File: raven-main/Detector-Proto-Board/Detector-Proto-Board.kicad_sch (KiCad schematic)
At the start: 17 parts, among them IC1 ADA4817-1ARDZ-R7, J1 Conn_01x04, U9 TLV3201AIDCKT

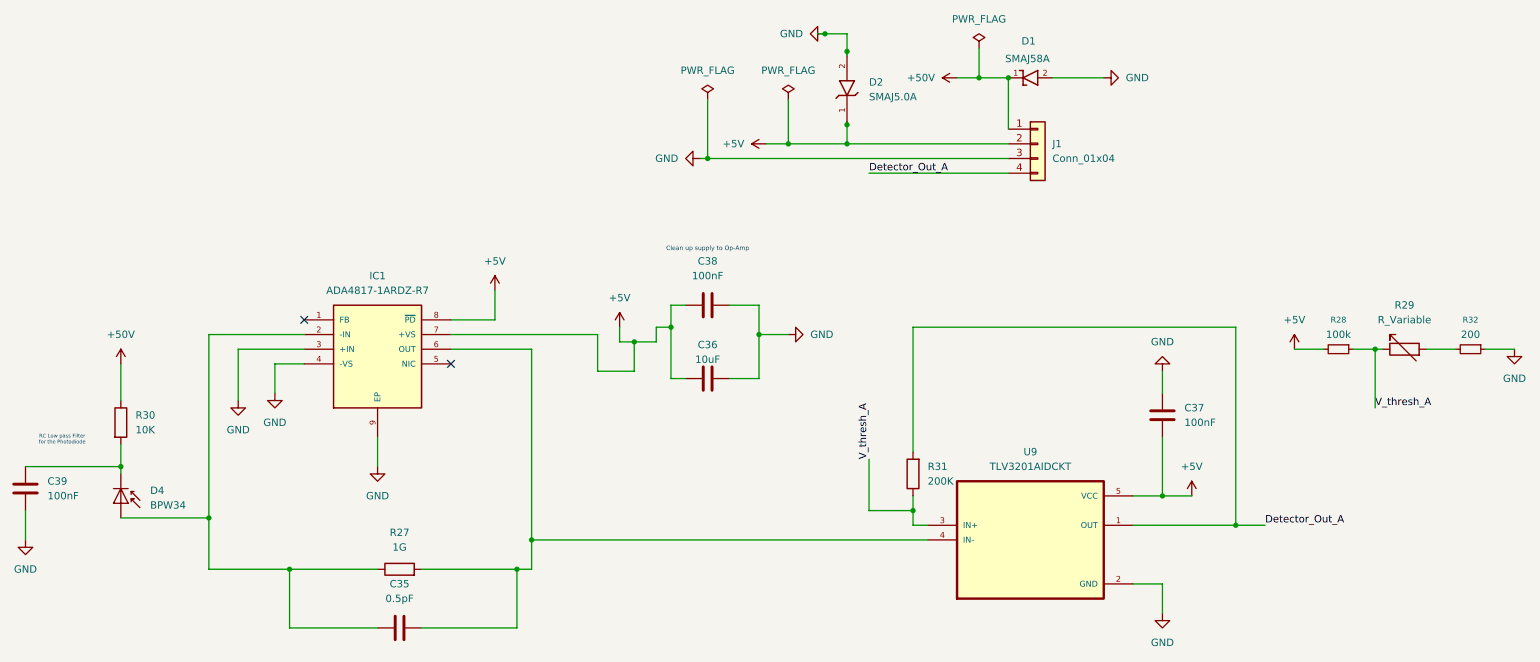
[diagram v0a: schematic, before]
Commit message: feat:PCB layout changes - example
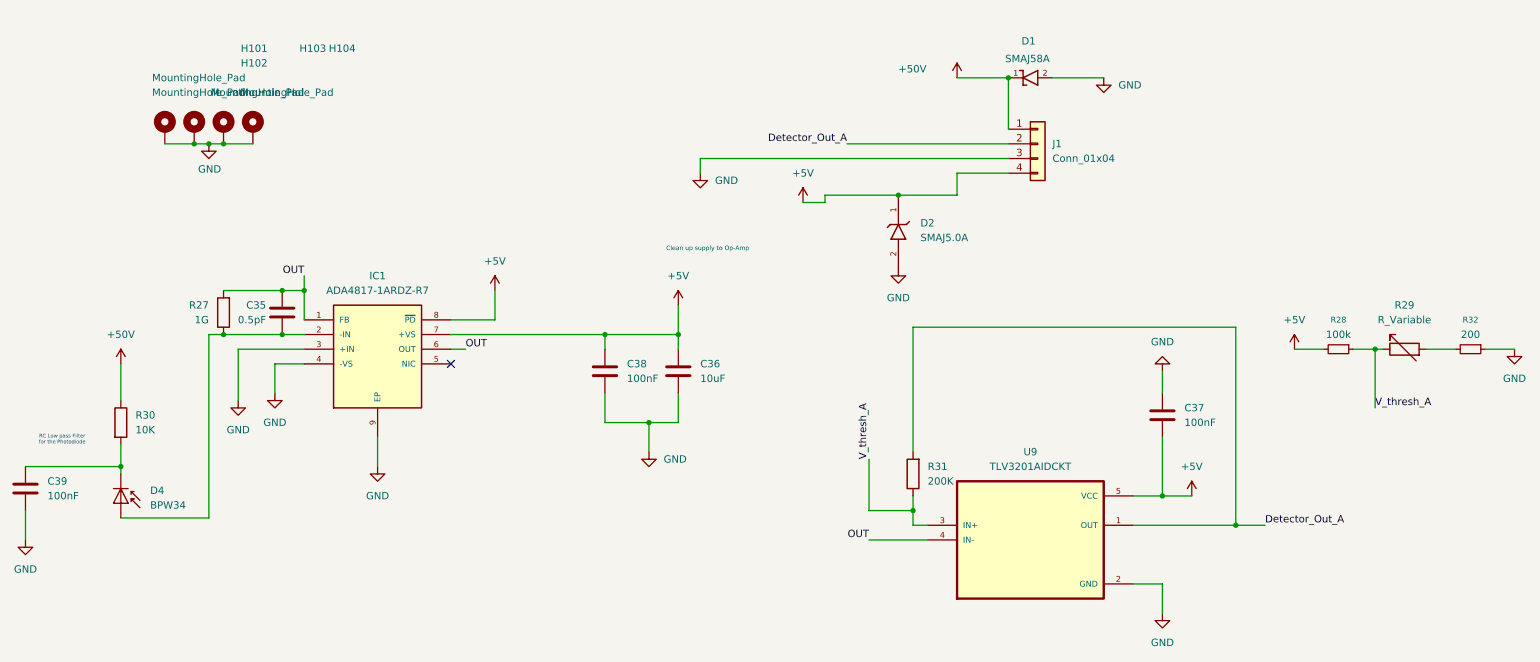
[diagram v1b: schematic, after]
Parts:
- added H101, H102, H103, H104: MountingHole_Pad, MountingHole:MountingHole_3.2mm_M3_DIN965_Pad, symbol Mechanical:MountingHole_Pad
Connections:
- net +5V: now also J1.4 (Pin_4); no longer J1.2 (Pin_2)
- net Detector_Out_A: now also J1.2 (Pin_2); no longer J1.4 (Pin_4)
- net GND: now also H101.1, H102.1, H103.1, H104.1
- net OUT: now reaches C35.2, IC1.6 (OUT), R27.2, U9.4 (IN-)
- net OUT: now also IC1.1 (FB)
- no-connect marks 2 -> 1
